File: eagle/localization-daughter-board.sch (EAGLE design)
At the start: 7 parts, among them U1 LM340MP-5.0/NOPB, U2 STM32F042FXP

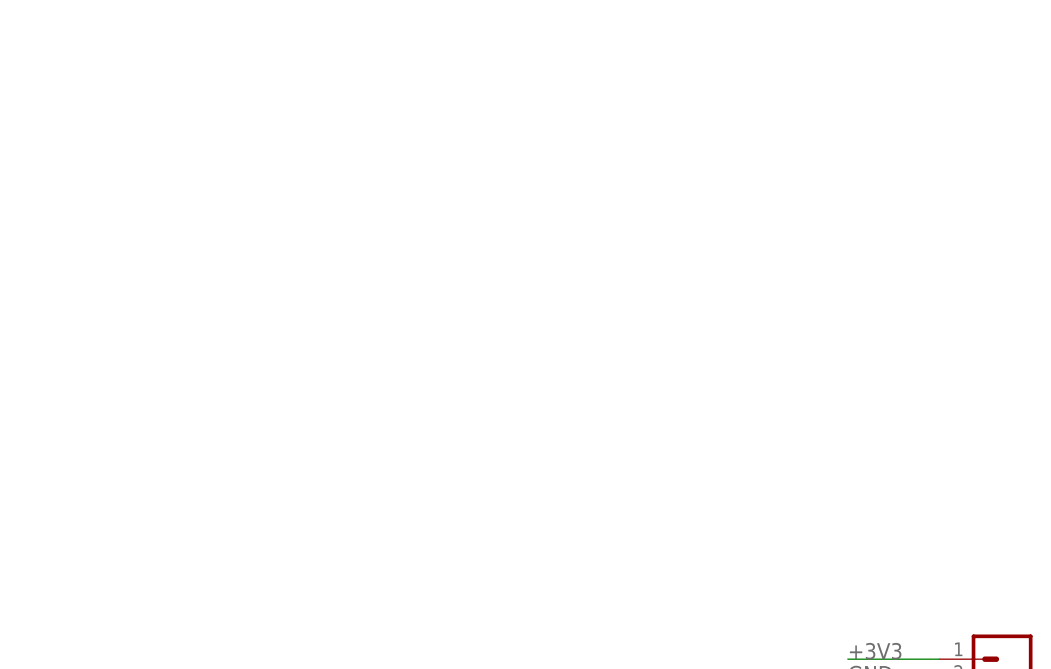
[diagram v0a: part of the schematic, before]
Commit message: Just saving progress
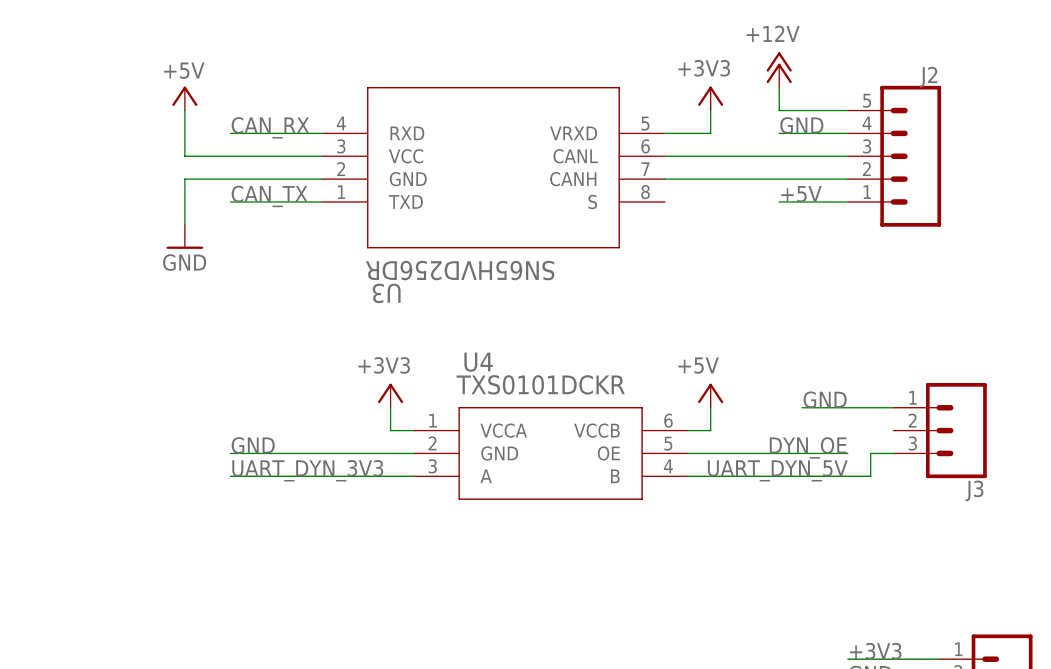
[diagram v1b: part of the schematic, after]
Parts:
- added J2: (no value), SparkFun-Connectors:CONN_05JST-VERT
- added J3: (no value), Localization-Daughter-Board:CONN_03
- added U3: SN65HVD256DR, Localization-Daughter-Board:SN65HVD256DR
- added U4: TXS0101DCKR, Localization-Daughter-Board:TXS0101DCKR
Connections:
- new net DYN_OE: U4.OE
- new net N$2: J2.2, U3.CANH
- new net N$3: J2.3, U3.CANL
- new net UART_DYN_3V3: U4.A
- new net UART_DYN_5V: J3.3, U4.B
- net +12V: now also J2.5
- net +3V3: now also U3.VRXD, U4.VCCA
- net +5V: now also J2.1, U3.VCC, U4.VCCB
- net CAN_RX: now also U3.RXD
- net CAN_TX: now also U3.TXD
- net GND: now also J2.4, J3.1, U3.GND, U4.GND
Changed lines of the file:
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@@
 <part name="GND3" library="supply1" library_urn="urn:adsk.eagle:library:371" deviceset="GND" device=""/>
 <part name="J1" library="SparkFun-Connectors" deviceset="CONN_05" device=""/>
+<part name="J2" library="SparkFun-Connectors" deviceset="CONN_05" device="JST-VERT"/>
+<part name="U3" library="Localization-Daughter-Board" library_urn="urn:adsk.eagle:library:1230207" deviceset="SN65HVD256DR" device=""/>
+<part name="+3V2" library="supply1" library_urn="urn:adsk.eagle:library:371" deviceset="+3V3" device=""/>
+<part name="P+5" library="supply1" library_urn="urn:adsk.eagle:library:371" deviceset="+5V" device=""/>
+<part name="GND5" library="supply1" library_urn="urn:adsk.eagle:library:371" deviceset="GND" device=""/>
+<part name="J3" library="Localization-Daughter-Board" library_urn="urn:adsk.eagle:library:1230207" deviceset="CONN_03" device=""/>
+<part name="U4" library="Localization-Daughter-Board" library_urn="urn:adsk.eagle:library:1230207" deviceset="TXS0101DCKR" device="" package3d_urn="urn:adsk.eagle:package:1230550/1"/>
+<part name="P+6" library="supply1" library_urn="urn:adsk.eagle:library:371" deviceset="+5V" device=""/>
+<part name="+3V3" library="supply1" library_urn="urn:adsk.eagle:library:371" deviceset="+3V3" device=""/>
+<part name="P+4" library="supply1" library_urn="urn:adsk.eagle:library:371" deviceset="+12V" device=""/>
 </parts>
 <sheets>
@@
 <instance part="GND3" gate="1" x="137.16" y="68.58"/>
 <instance part="J1" gate="G$1" x="254" y="116.84" rot="R180"/>
+<instance part="J2" gate="G$1" x="243.84" y="177.8" rot="MR0"/>
+<instance part="U3" gate="A" x="175.26" y="172.72" rot="MR180"/>
+<instance part="+3V2" gate="G$1" x="220.98" y="185.42" smashed="yes">
+<attribute name="VALUE" x="217.17" y="186.69" size="1.778" layer="96"/>
+</instance>
+<instance part="P+5" gate="1" x="162.56" y="185.42" smashed="yes">
+<attribute name="VALUE" x="160.02" y="186.436" size="1.778" layer="96"/>
+</instance>
+<instance part="GND5" gate="1" x="162.56" y="167.64"/>
+<instance part="J3" gate="G$1" x="248.92" y="147.32" rot="R180"/>
+<instance part="U4" gate="A" x="185.42" y="147.32"/>
+<instance part="P+6" gate="1" x="220.98" y="152.4" smashed="yes">
+<attribute name="VALUE" x="217.17" y="153.67" size="1.778" layer="96"/>
+</instance>
+<instance part="+3V3" gate="G$1" x="185.42" y="152.4" smashed="yes">
+<attribute name="VALUE" x="181.61" y="153.67" size="1.778" layer="96"/>
+</instance>
+<instance part="P+4" gate="1" x="228.6" y="187.96" smashed="yes">
+<attribute name="VALUE" x="230.886" y="190.5" size="1.778" layer="96" rot="MR0"/>
+</instance>
 </instances>
 <busses>
@@
 <pinref part="U1" gate="A" pin="IN"/>
 <wire x1="48.26" y1="137.16" x2="50.8" y2="137.16" width="0.1524" layer="91"/>
+</segment>
+<segment>
+<pinref part="J2" gate="G$1" pin="5"/>
+<wire x1="236.22" y1="182.88" x2="228.6" y2="182.88" width="0.1524" layer="91"/>
+<pinref part="P+4" gate="1" pin="+12V"/>
+<wire x1="228.6" y1="182.88" x2="228.6" y2="185.42" width="0.1524" layer="91"/>
 </segment>
 </net>
@@
 <label x="236.22" y="119.38" size="1.778" layer="95"/>
 </segment>
+<segment>
+<pinref part="GND5" gate="1" pin="GND"/>
+<wire x1="162.56" y1="170.18" x2="162.56" y2="175.26" width="0.1524" layer="91"/>
+<pinref part="U3" gate="A" pin="GND"/>
+<wire x1="177.8" y1="175.26" x2="162.56" y2="175.26" width="0.1524" layer="91"/>
+</segment>
+<segment>
+<pinref part="J3" gate="G$1" pin="1"/>
+<wire x1="241.3" y1="149.86" x2="231.14" y2="149.86" width="0.1524" layer="91"/>
+<label x="236.22" y="149.86" size="1.778" layer="95" rot="MR0"/>
+</segment>
+<segment>
+<pinref part="U4" gate="A" pin="GND"/>
+<wire x1="187.96" y1="144.78" x2="167.64" y2="144.78" width="0.1524" layer="91"/>
+<label x="167.64" y="144.78" size="1.778" layer="95"/>
+</segment>
+<segment>
+<pinref part="J2" gate="G$1" pin="4"/>
+<wire x1="236.22" y1="180.34" x2="228.6" y2="180.34" width="0.1524" layer="91"/>
+<label x="228.6" y="180.34" size="1.778" layer="95"/>
+</segment>
 </net>
 <net name="+5V" class="0">
@@
 <junction x="99.06" y="78.74"/>
 </segment>
+<segment>
+<pinref part="P+5" gate="1" pin="+5V"/>
+<wire x1="162.56" y1="182.88" x2="162.56" y2="177.8" width="0.1524" layer="91"/>
+<pinref part="U3" gate="A" pin="VCC"/>
+<wire x1="177.8" y1="177.8" x2="162.56" y2="177.8" width="0.1524" layer="91"/>
+</segment>
+<segment>
+<pinref part="U4" gate="A" pin="VCCB"/>
+<wire x1="218.44" y1="147.32" x2="220.98" y2="147.32" width="0.1524" layer="91"/>
+<pinref part="P+6" gate="1" pin="+5V"/>
+<wire x1="220.98" y1="149.86" x2="220.98" y2="147.32" width="0.1524" layer="91"/>
+</segment>
+<segment>
+<pinref part="J2" gate="G$1" pin="1"/>
+<wire x1="236.22" y1="172.72" x2="228.6" y2="172.72" width="0.1524" layer="91"/>
+<label x="228.6" y="172.72" size="1.778" layer="95"/>
+</segment>
 </net>
 <net name="+3V3" class="0">
@@
 <wire x1="246.38" y1="121.92" x2="236.22" y2="121.92" width="0.1524" layer="91"/>
 <label x="236.22" y="121.92" size="1.778" layer="95"/>
+</segment>
+<segment>
+<pinref part="U3" gate="A" pin="VRXD"/>
+<wire x1="215.9" y1="180.34" x2="220.98" y2="180.34" width="0.1524" layer="91"/>
+<pinref part="+3V2" gate="G$1" pin="+3V3"/>
+<wire x1="220.98" y1="180.34" x2="220.98" y2="182.88" width="0.1524" layer="91"/>
+</segment>
+<segment>
+<pinref part="U4" gate="A" pin="VCCA"/>
+<wire x1="187.96" y1="147.32" x2="185.42" y2="147.32" width="0.1524" layer="91"/>
+<pinref part="+3V3" gate="G$1" pin="+3V3"/>
+<wire x1="185.42" y1="149.86" x2="185.42" y2="147.32" width="0.1524" layer="91"/>
 </segment>
 </net>
@@
 <label x="231.14" y="88.9" size="1.778" layer="95" rot="MR0"/>
 </segment>
+<segment>
+<pinref part="U3" gate="A" pin="TXD"/>
+<wire x1="177.8" y1="172.72" x2="167.64" y2="172.72" width="0.1524" layer="91"/>
+<label x="167.64" y="172.72" size="1.778" layer="95"/>
+</segment>
 </net>
 <net name="CAN_RX" class="0">
@@
 <label x="231.14" y="86.36" size="1.778" layer="95" rot="MR0"/>
 </segment>
+<segment>
+<pinref part="U3" gate="A" pin="RXD"/>
+<wire x1="177.8" y1="180.34" x2="167.64" y2="180.34" width="0.1524" layer="91"/>
+<label x="167.64" y="180.34" size="1.778" layer="95"/>
+</segment>
 </net>
 <net name="SDA1" class="0">
@@
 </segment>
 </net>
+<net name="N$2" class="0">
+<segment>
+<pinref part="J2" gate="G$1" pin="2"/>
+<pinref part="U3" gate="A" pin="CANH"/>
+<wire x1="236.22" y1="175.26" x2="215.9" y2="175.26" width="0.1524" layer="91"/>
+</segment>
+</net>
+<net name="N$3" class="0">
+<segment>
+<pinref part="J2" gate="G$1" pin="3"/>
+<pinref part="U3" gate="A" pin="CANL"/>
+<wire x1="236.22" y1="177.8" x2="215.9" y2="177.8" width="0.1524" layer="91"/>
+</segment>
+</net>
+<net name="UART_DYN_5V" class="0">
+<segment>
+<pinref part="J3" gate="G$1" pin="3"/>
+<wire x1="241.3" y1="144.78" x2="238.76" y2="144.78" width="0.1524" layer="91"/>
+<label x="236.22" y="142.24" size="1.778" layer="95" rot="MR0"/>
+<pinref part="U4" gate="A" pin="B"/>
+<wire x1="218.44" y1="142.24" x2="238.76" y2="142.24" width="0.1524" layer="91"/>
+<wire x1="238.76" y1="142.24" x2="238.76" y2="144.78" width="0.1524" layer="91"/>
+</segment>
+</net>
+<net name="DYN_OE" class="0">
+<segment>
+<pinref part="U4" gate="A" pin="OE"/>
+<wire x1="218.44" y1="144.78" x2="236.22" y2="144.78" width="0.1524" layer="91"/>
+<label x="236.22" y="144.78" size="1.778" layer="95" rot="MR0"/>
+</segment>
+</net>
+<net name="UART_DYN_3V3" class="0">
+<segment>
+<pinref part="U4" gate="A" pin="A"/>
+<wire x1="187.96" y1="142.24" x2="167.64" y2="142.24" width="0.1524" layer="91"/>
+<label x="167.64" y="142.24" size="1.778" layer="95"/>
+</segment>
+</net>
